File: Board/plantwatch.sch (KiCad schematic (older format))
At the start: 27 parts, among them J3 SWD Connector, J4 Jack-DC, SW1 SW_Push, SW2 SW_Push, U1 MKL25Z128VLK4, U4 NCP1117-3.3_SOT223, Y1 Crystal_GND24

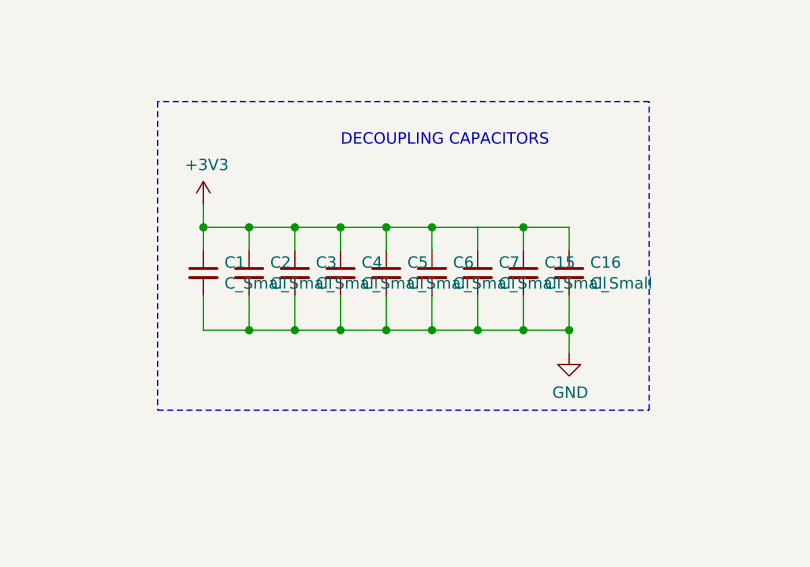
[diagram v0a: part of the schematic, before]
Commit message: Make layout
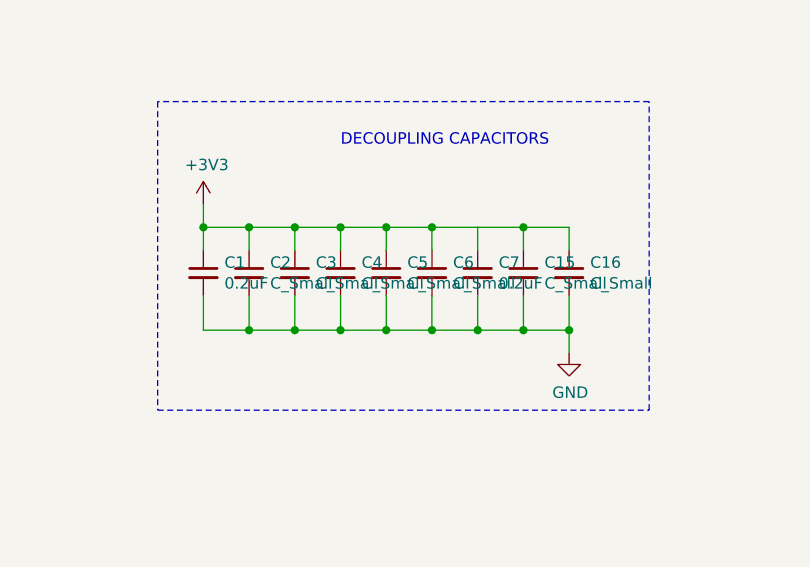
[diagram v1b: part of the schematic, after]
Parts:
- C1, C7: value C_Small -> 0.2uF
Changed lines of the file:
@@
 P 8400 1550
 F 0 "C1" H 8492 1596 50  0000 L CNN
-F 1 "C_Small" H 8492 1505 50  0000 L CNN
+F 1 "0.2uF" H 8492 1505 50  0000 L CNN
 F 2 "Capacitor_THT:CP_Radial_Tantal_D4.5mm_P5.00mm" H 8400 1550 50  0001 C CNN
 F 3 "~" H 8400 1550 50  0001 C CNN
@@
 P 9600 1550
 F 0 "C7" H 9692 1596 50  0000 L CNN
-F 1 "C_Small" H 9692 1505 50  0000 L CNN
+F 1 "0.2uF" H 9692 1505 50  0000 L CNN
 F 2 "Capacitor_THT:CP_Radial_Tantal_D4.5mm_P5.00mm" H 9600 1550 50  0001 C CNN
 F 3 "~" H 9600 1550 50  0001 C CNN
@@
 	9800 1800 9600 1800
 Wire Wire Line
+	9800 1350 9800 1450
+Connection ~ 10000 1800
+Wire Wire Line
 	9600 1350 9800 1350
-Wire Wire Line
-	9800 1350 9800 1450
 Connection ~ 9800 1350
 Wire Wire Line
 	9800 1350 10000 1350
-Connection ~ 10000 1800
 $EndSCHEMATC
